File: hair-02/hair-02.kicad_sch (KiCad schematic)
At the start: 20 parts, among them J1 TYPE-C-31-M-12, U1 ESP32-C3-WROOM-02, U2 AP2112K-3.3, U3 TSMP58000

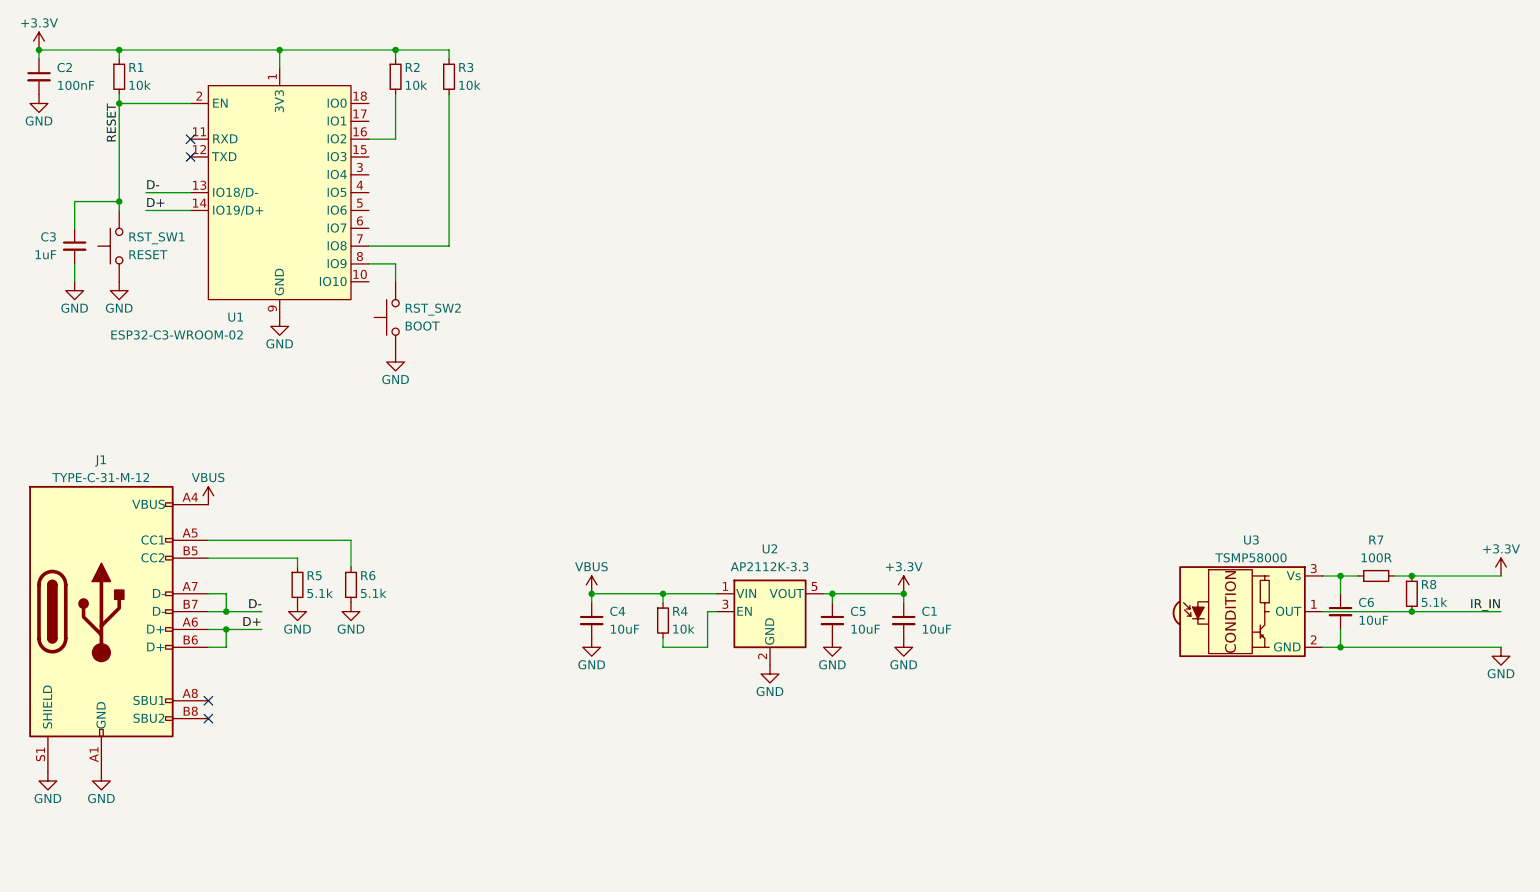
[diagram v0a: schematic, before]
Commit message: hair-02: Component selection and schematic done
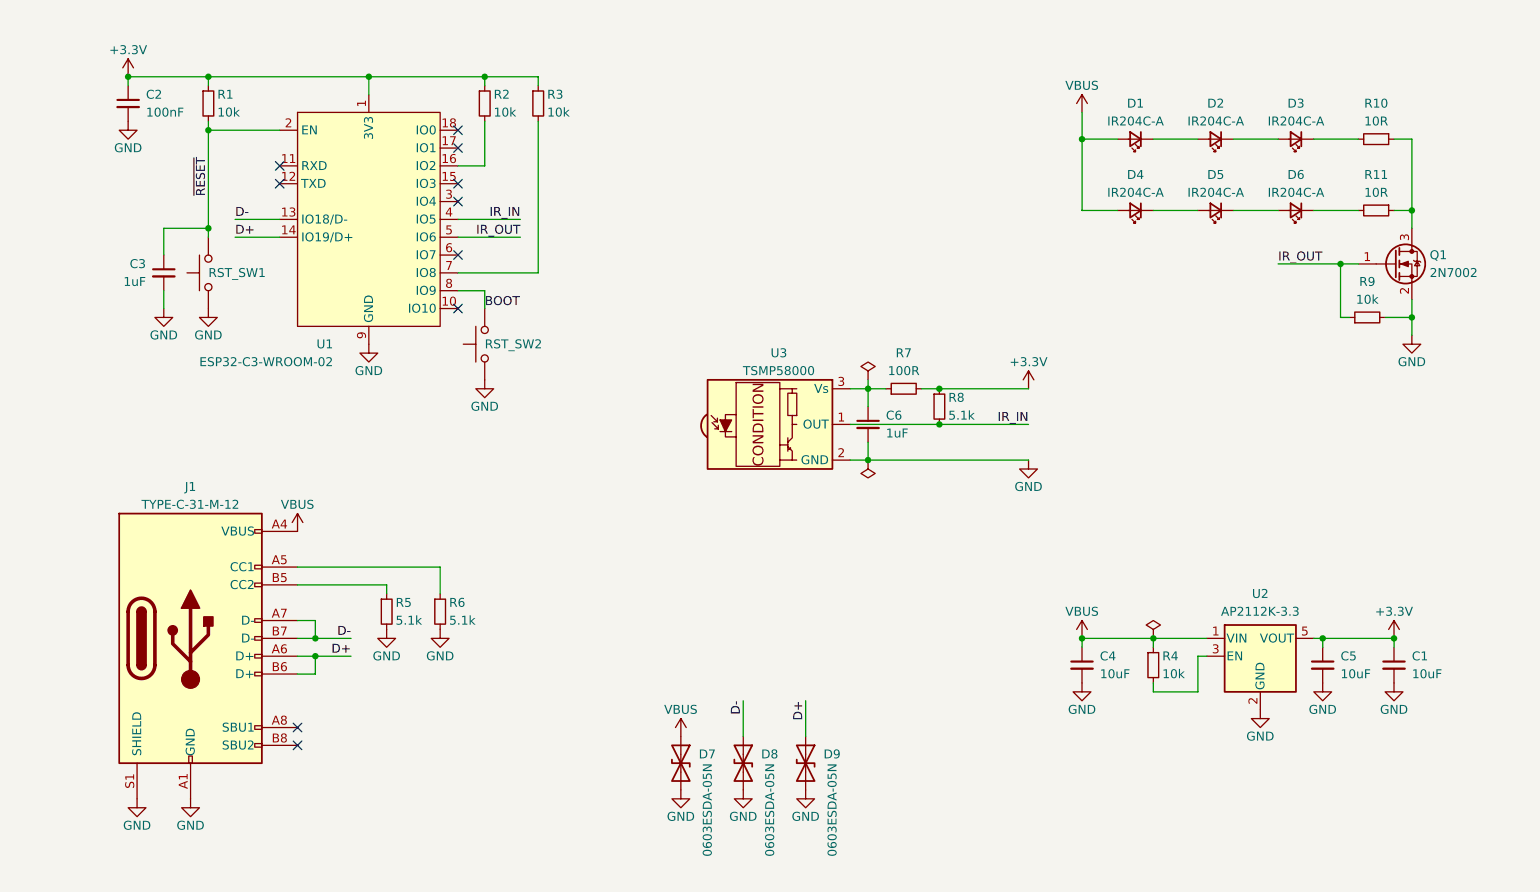
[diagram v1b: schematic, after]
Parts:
- added D1, D2, D3, D4, D5, D6: IR204C-A, LED_THT:LED_D3.0mm, symbol Device:LED_Small
- added D7, D8, D9: 0603ESDA-05N, Diode_SMD:D_0603_1608Metric, symbol Device:D_TVS
- added Q1: 2N7002, Package_TO_SOT_SMD:SOT-23, symbol Transistor_FET:2N7002
- added R10, R11: 10R, Resistor_SMD:R_1206_3216Metric, symbol Device:R_Small
- added R9: 10k, Resistor_SMD:R_0603_1608Metric, symbol Device:R_Small
- C3: footprint (none) -> Capacitor_SMD:C_0805_2012Metric; LCSC (none) -> C28323
- C6: value 10uF -> 1uF; footprint Capacitor_SMD:C_1206_3216Metric -> Capacitor_SMD:C_0805_2012Metric; LCSC C13585 -> C28323
- RST_SW1: value RESET -> SKRK
- RST_SW2: value BOOT -> SKRK
- U1: LCSC (none) -> C2934560
- U3: footprint hair-01:Vishay_MINICAST-3Pin-SMD -> OptoDevice:Vishay_MINICAST-3Pin
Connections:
- net D+: now also D9.1 (A1)
- net D-: now also D8.1 (A1)
- net GND: now also D7.2 (A2), D8.2 (A2), D9.2 (A2), Q1.2 (S), R9.2
- net IR_IN: now also U1.4 (IO5)
- net VBUS: now also D1.2 (A), D4.2 (A), D7.1 (A1)
- net IR_OUT: now reaches U1.5 (IO6)
- net IR_OUT: now also Q1.1 (G), R9.1
- net BOOT: now reaches RST_SW2.2, U1.8 (IO9)
- net RESET renamed ~{RESET}
- new net: D3.1 (K), R10.2
- new net: D2.1 (K), D3.2 (A)
- new net: D4.1 (K), D5.2 (A)
- new net: Q1.3 (D), R10.1, R11.1
- new net: D1.1 (K), D2.2 (A)
- new net: D6.1 (K), R11.2
- new net: D5.1 (K), D6.2 (A)
- no-connect marks 4 -> 10
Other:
- moved on the sheet: C1, C2, C3, C4, C5, J1, R1, R2, R3, R4, R5, R6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

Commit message: hair-02: Implement ESP32-C3-WROOM-02 footprint
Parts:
- U1: footprint (none) -> hair-02:ESP32-C3-WROOM-02
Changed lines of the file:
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@@
       (effects (font (size 1.27 1.27)) (justify right))
     )
-    (property "Footprint" "" (id 2) (at 103.505 80.645 0)
+    (property "Footprint" "hair-02:ESP32-C3-WROOM-02" (id 2) (at 103.505 80.645 0)
       (effects (font (size 1.27 1.27)) hide)
     )
@@
     )
     (path "/13726d9d-fbe1-483a-84a4-1b1ebec6db05"
-      (reference "U1") (unit 1) (value "ESP32-C3-WROOM-02") (footprint "")
+      (reference "U1") (unit 1) (value "ESP32-C3-WROOM-02") (footprint "hair-02:ESP32-C3-WROOM-02")
     )
     (path "/e6669ec5-528f-4678-b381-e1890d50919a"
